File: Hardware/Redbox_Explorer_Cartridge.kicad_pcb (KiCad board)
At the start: 2 copper layers, 49.8 x 63.2 mm, 59 parts, among them Q1 BS170, Q10 BS170, Q11 BS170, Q12 BS170, Q13 BS170, Q14 BS170, Q15 BS170, Q2 BS170, Q3 BS170, Q4 BS170, Q5 BS170, Q6 BS170, Q7 BS170, Q8 BS170, Q9 BS170, U1 MCP3008

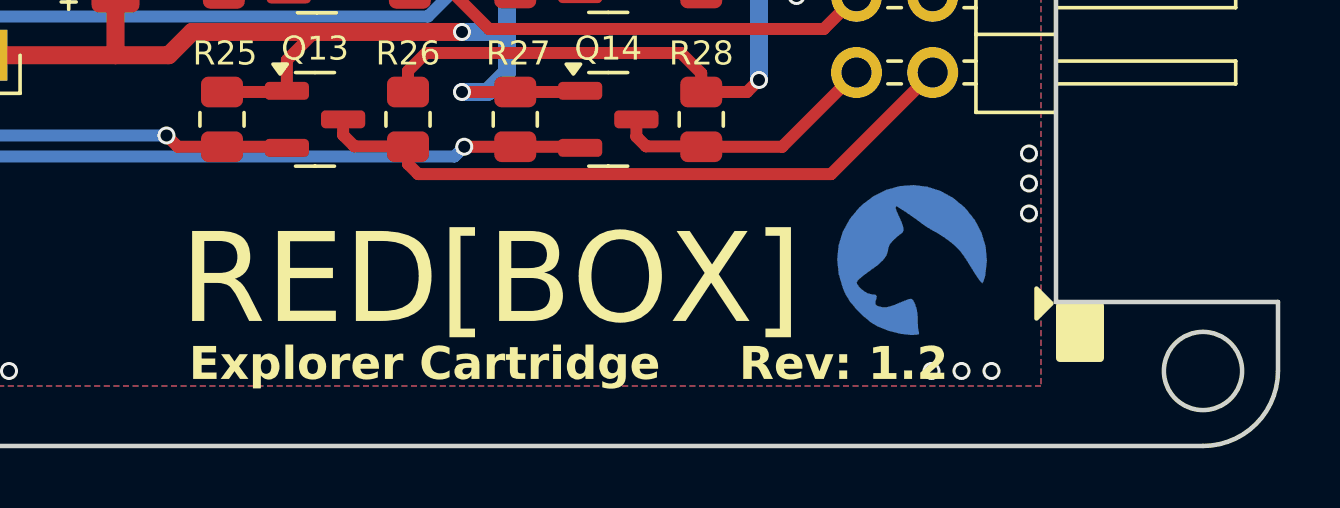
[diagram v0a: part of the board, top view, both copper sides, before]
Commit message: Brand colors update
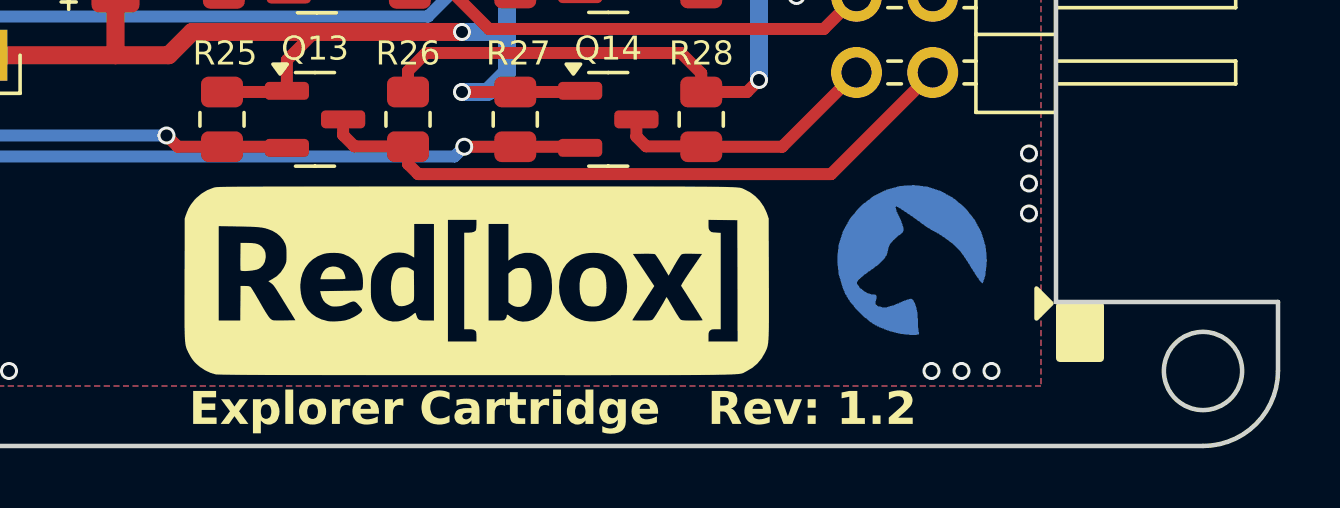
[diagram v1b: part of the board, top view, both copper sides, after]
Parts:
- added G***: LOGO, LOGO, F.Cu at (148.3, 129.5)
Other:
- board text removed: "RED[BOX]"
